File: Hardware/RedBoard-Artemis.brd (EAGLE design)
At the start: 68.6 x 53.3 mm, 112 parts, among them IC3 LM1117, J2 CORTEX_DEBUG, J3 POWER_JACKTOE, J5 USB-C, Q1 1.1A/60V/600mΩ, U1 ARTEMIS_MODULESMD, U3 AP2112-3.3V, U5 CH340C, Y1 32.768kHz

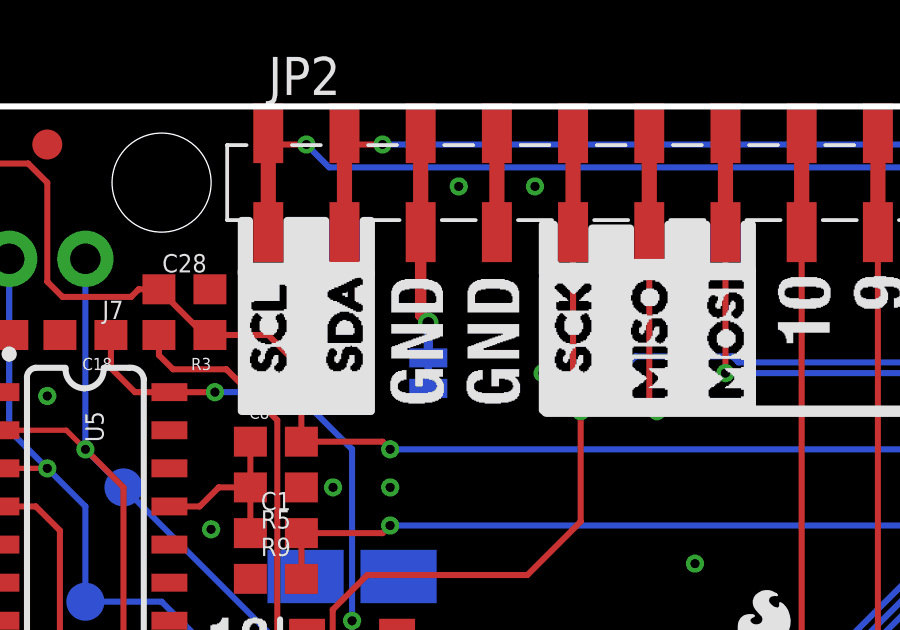
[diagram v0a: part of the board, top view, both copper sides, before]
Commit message: Silk adjust
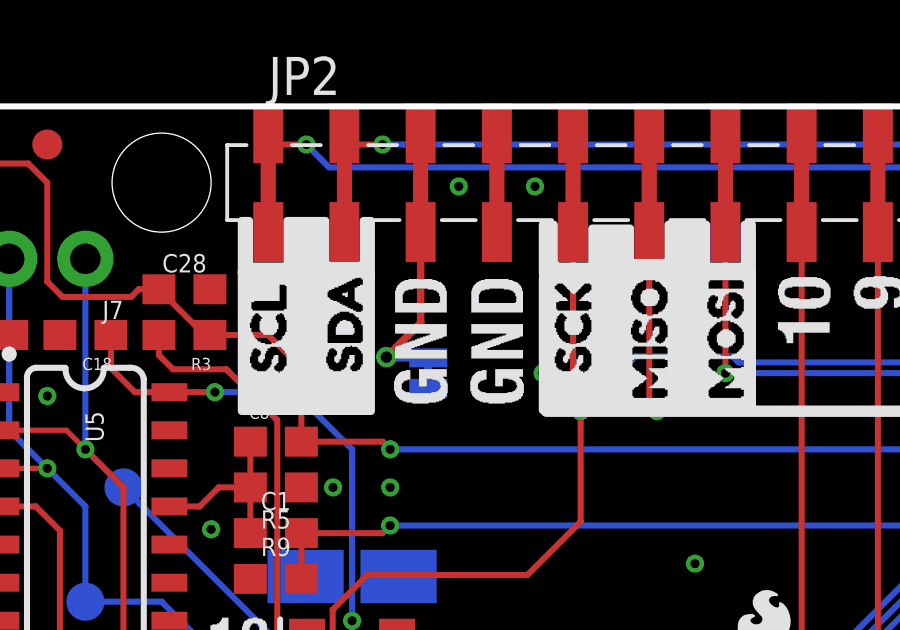
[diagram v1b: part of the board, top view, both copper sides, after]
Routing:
- net N$10: track 7.60 -> 9.35 mm
